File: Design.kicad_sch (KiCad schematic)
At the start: 41 parts, among them J1 Conn_02x16_Odd_Even, J2 Conn_01x01_Pin, J3 Conn_01x01_Pin, J4 Conn_01x02_Pin, J5 Conn_01x02, Q1 DMP3099L, Q2 2N7002, Q3 SI2301CDS-T1-GE3, U1 AMS1117, U2 INA219AIDCNR, U3 TP4056, U4 TPS54331DR, U5 DRV8833PWP, U6 MT3608L, U7 TPS54331DR

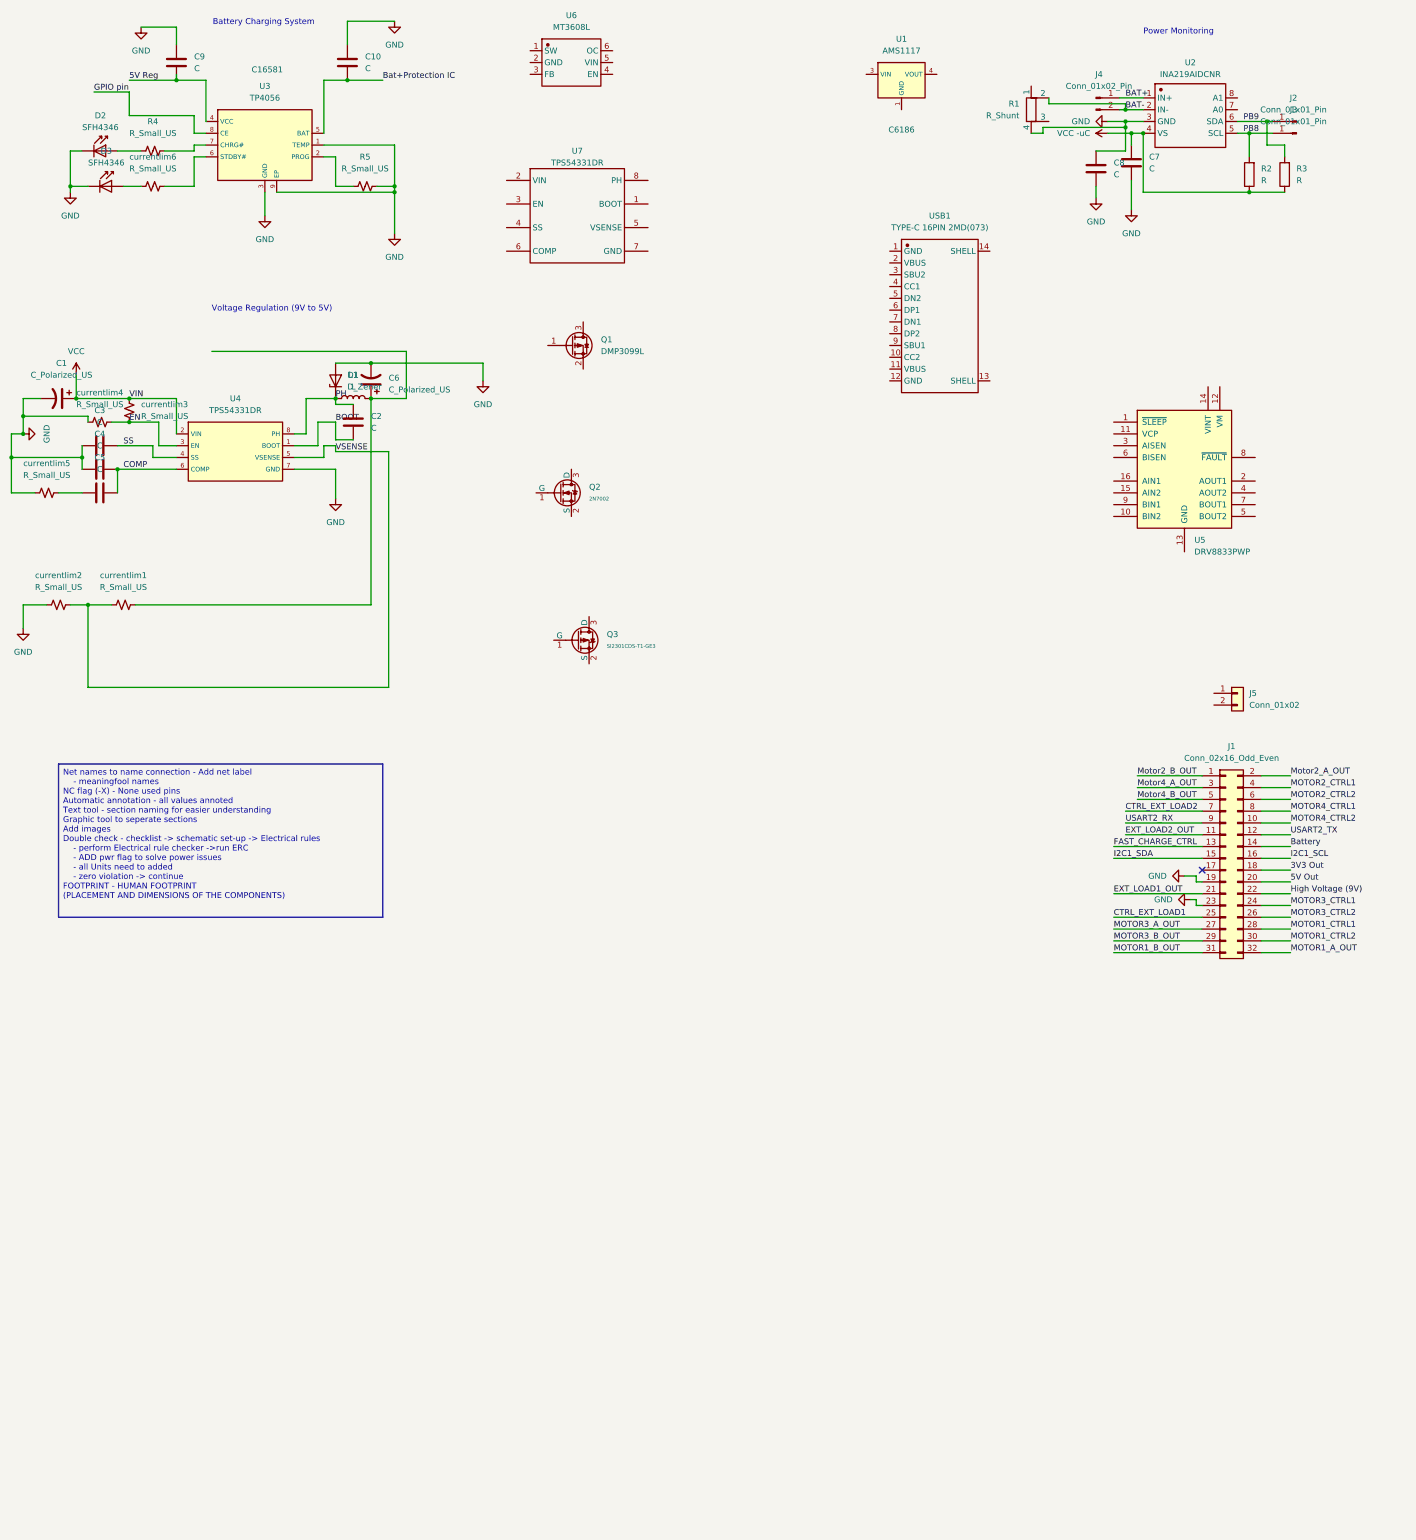
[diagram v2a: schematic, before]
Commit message: Add files via upload
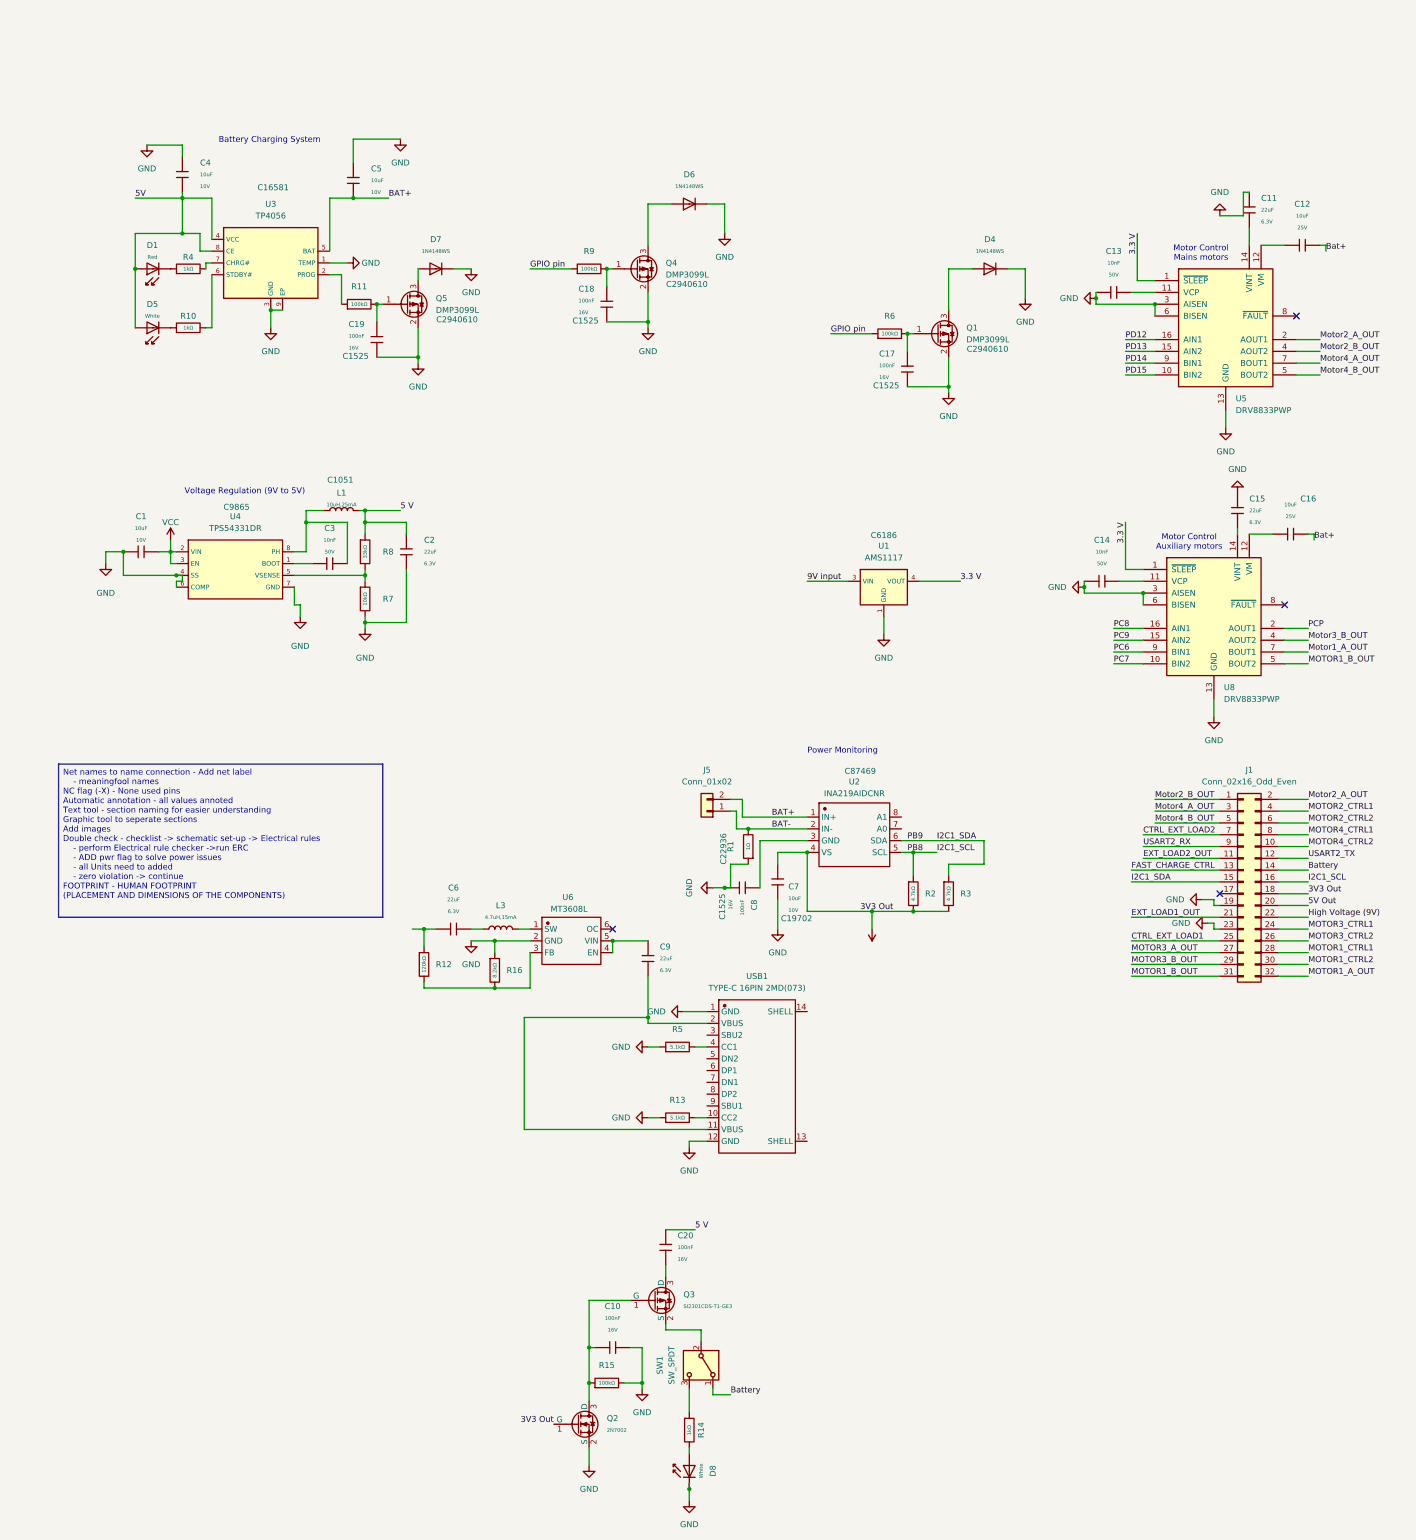
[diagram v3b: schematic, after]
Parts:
- removed C1, C6: C_Polarized_US, symbol Device:C_Polarized_US
- removed C10, C2, C3, C4, C5, C7, C8, C9: C, symbol Device:C
- removed D1: D_Zener, symbol Device:D_Zener
- removed D2, D3: SFH4346, LED_THT:LED_D3.0mm_IRBlack, symbol LED:SFH4346
- removed J2, J3: Conn_01x01_Pin, symbol Connector:Conn_01x01_Pin
- removed J4: Conn_01x02_Pin, symbol Connector:Conn_01x02_Pin
- removed L1: L, symbol Device:L
- removed R1: R_Shunt, symbol Device:R_Shunt
- removed R2, R3: R, symbol Device:R
- removed R4, R5, currentlim1, currentlim2, currentlim3, currentlim4, currentlim5, currentlim6: R_Small_US, symbol Device:R_Small_US
- removed U7: TPS54331DR, symbol SCHLIB_TPS54331DR_2025-03-24:TPS54331DR
- added C1, C4, C5, C7: 10uF, PCM_JLCPCB:C_0603, symbol PCM_JLCPCB-Capacitors:0603,10uF
- added C10, C17, C18, C19, C20, C8: 100nF, PCM_JLCPCB:C_0402, symbol PCM_JLCPCB-Capacitors:0402,100nF
- added C11, C15, C2, C6, C9: 22uF, PCM_JLCPCB:C_0603, symbol PCM_JLCPCB-Capacitors:0603,22uF
- added C12, C16: 10uF, PCM_JLCPCB:C_0805, symbol PCM_JLCPCB-Capacitors:0805,10uF
- added C13, C14, C3: 10nF, PCM_JLCPCB:C_0402, symbol PCM_JLCPCB-Capacitors:0402,10nF
- added D1: Red, PCM_JLCPCB:D_0603, symbol PCM_JLCPCB-Diodes:LED,0603,Red
- added D4, D6, D7: 1N4148WS, PCM_JLCPCB:D_SOD-323, symbol PCM_JLCPCB-Diodes:Switching,1N4148WS
- added D5, D8: White, PCM_JLCPCB:D_0603, symbol PCM_JLCPCB-Diodes:LED,0603,White
- added L1: 10uH,25mA, PCM_JLCPCB:L_1206, symbol PCM_JLCPCB-Inductors:10uH,25mA
- added L3: 4.7uH,15mA, PCM_JLCPCB:L_0603, symbol PCM_JLCPCB-Inductors:4.7uH,15mA
- added Q4, Q5: DMP3099L, PCM_JLCPCB:SOT-23-3_L2.9-W1.3-P0.95-LS2.4-BR, symbol Transistor_FET:DMP3099L
- added R1: 1Ω, PCM_JLCPCB:R_0603, symbol PCM_JLCPCB-Resistors:0603,1Ω
- added R10, R14, R4: 1kΩ, PCM_JLCPCB:R_0402, symbol PCM_JLCPCB-Resistors:0402,1kΩ
- added R11, R15, R6, R9: 100kΩ, PCM_JLCPCB:R_0603, symbol PCM_JLCPCB-Resistors:0603,100kΩ
- added R12: 120kΩ, PCM_JLCPCB:R_0402, symbol PCM_JLCPCB-Resistors:0402,120kΩ
- added R13, R5: 5.1kΩ, PCM_JLCPCB:R_0402, symbol PCM_JLCPCB-Resistors:0402,5.1kΩ
- added R16: 8.2kΩ, PCM_JLCPCB:R_0402, symbol PCM_JLCPCB-Resistors:0402,8.2kΩ
- added R2, R3: 4.7kΩ, PCM_JLCPCB:R_0402, symbol PCM_JLCPCB-Resistors:0402,4.7kΩ
- added R7: 10kΩ, PCM_JLCPCB:R_0402, symbol PCM_JLCPCB-Resistors:0402,10kΩ
- added R8: 33kΩ, PCM_JLCPCB:R_0402, symbol PCM_JLCPCB-Resistors:0402,33kΩ
- added SW1: SW_SPDT, symbol Switch:SW_SPDT
- added U8: DRV8833PWP, Package_SO:HTSSOP-16-1EP_4.4x5mm_P0.65mm_EP3.4x5mm_Mask2.46x2.31mm_ThermalVias, symbol Driver_Motor:DRV8833PWP
- Q1: Part (none) -> C2940610
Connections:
- net Bat+Protection IC is gone; now on net BAT+: U3.5 (BAT)
- net COMP is gone; now on net GND: U4.6 (COMP)
- net EN is gone; now on net VCC: U4.3 (EN)
- net PB8 is gone; now on net I2C1_SCL: U2.5 (SCL)
- net PB9 is gone; now on net I2C1_SDA : U2.6 (SDA)
- net SS is gone; now on net GND: U4.4 (SS)
- net VCC -uC is gone; now on net 3V3 Out : U2.4 (VS)
- net 3V3 Out : now also Q2.1 (G), C7.1, R2.2, R3.2
- net BAT+: now also J5.2 (Pin_2), C5.2
- net BAT-: now also J5.1 (Pin_1), R1.2
- net Battery : now also SW1.1 (A)
- net GND: now also Q1.2 (S), Q2.2 (S), U1.1 (GND), U5.13 (GND), U5.17 (GND), U5.3 (AISEN), U5.6 (BISEN), U6.2 (GND), USB1.1 (GND), USB1.12 (GND), C1.1, C10.2, C11.1, C13.1, C14.1, C15.1, C17.2, C18.2, C19.2, C2.2, C4.1, C5.1, C7.2, C8.2, D4.1, D6.1, D7.1, D8.1, Q4.2 (S), Q5.2 (S), R1.1, R13.1, R15.2, R16.1, R5.1, R7.2, U8.13 (GND), U8.17 (GND), U8.3 (AISEN), U8.6 (BISEN); no longer U2.3 (GND)
- net GPIO pin: now also R6.1, R9.1; no longer U3.8 (CE)
- net I2C1_SCL: now also R2.1
- net I2C1_SDA : now also R3.1
- net Motor2_A_OUT : now also U5.2 (AOUT1)
- net Motor2_B_OUT: now also U5.4 (AOUT2)
- net Motor4_A_OUT : now also U5.7 (BOUT1)
- net Motor4_B_OUT: now also U5.5 (BOUT2)
- net VCC: now also C1.2
- net at Q3.1 (G): now also Q2.3 (D), C10.1, R15.1
- net at Q3.2 (S): now also SW1.2 (B)
- net at Q3.3 (D): now also C20.1
- net 3.3 V: now reaches U5.1 (~{SLEEP})
- net 3.3 V: now also U1.2 (VOUT), U1.4 (VOUT), U8.1 (~{SLEEP})
- net PD15: now reaches U5.10 (BIN2)
- net at U5.11 (VCP): now also C13.2
- net at U5.12 (VM): now also C12.1
- net at U5.14 (VINT): now also C11.2
- net PD13: now reaches U5.15 (AIN2)
- net PD12: now reaches U5.16 (AIN1)
- net PD14: now reaches U5.9 (BIN1)
- net at U3.7 (CHRG#): now also R4.2
- net at USB1.10 (CC2): now also R13.2
- net at USB1.11 (VBUS): now also USB1.2 (VBUS), C9.1
- net at USB1.4 (CC1): now also R5.2
- net at U3.6 (STDBY#): now also R10.2
- net at U3.2 (PROG): now also R11.1
- net at Q1.1 (G): now also C17.1, R6.2
- net at Q1.3 (D): now also D4.2
- net 9V input: now reaches U1.3 (VIN)
- net at U6.1 (SW): now also L3.2
- net at U6.3 (FB): now also R12.2, R16.2
- net at U6.4 (EN): now also U6.5 (VIN), C9.2
- net 5V Reg renamed 5V 
- net 5V : now also U3.8 (CE), C4.2, D1.2, D5.2
- net BOOT: no longer names the net of U4.1 (BOOT)
- net BOOT: now also C3.1
- net PH: no longer names the net of U4.8 (PH)
- net PH: now also C3.2, L1.1
- net VSENSE: no longer names the net of U4.5 (VSENSE)
- net VSENSE: now also R7.1, R8.2
- new net: C18.1, Q4.1 (G), R9.2
- new net: D7.2, Q5.3 (D)
- new net: C16.1, U8.12 (VM)
- new net: C19.1, Q5.1 (G), R11.2
- new net: C8.1, U2.3 (GND)
- new net: C6.1, R12.1
- new net: C6.2, L3.1
- new net: D1.1, R4.1
- new net: R14.1, SW1.3 (C)
- new net: C14.2, U8.11 (VCP)
- new net: D8.2, R14.2
- new net: C15.2, U8.14 (VINT)
- new net: D5.1, R10.1
- new net: D6.2, Q4.3 (D)
- new net 5 V: C2.1, C20.2, L1.2, R8.1
- new net Bat+: C12.2, C16.2
- new net MOTOR1_B_OUT: U8.5 (BOUT2)
- new net Motor1_A_OUT : U8.7 (BOUT1)
- new net Motor3_B_OUT: U8.4 (AOUT2)
- new net PC6: U8.9 (BIN1)
- new net PC7: U8.10 (BIN2)
- new net PC8: U8.16 (AIN1)
- new net PC9: U8.15 (AIN2)
- new net PCP: U8.2 (AOUT1)
- no-connect marks 1 -> 4
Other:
- note added: "Motor Control Auxiliary motors"
- note added: "Motor Control Mains motors"
- moved on the sheet: J1, J5, Q1, Q2, Q3, U1, U2, U3, U4, U5, U6, USB1
